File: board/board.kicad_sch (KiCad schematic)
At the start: 13 parts, among them J1 Conn_01x19, J2 Conn_01x19, J3 Conn_01x02, U1 ESP32-WROVER-E, U2 AOZ1280CI

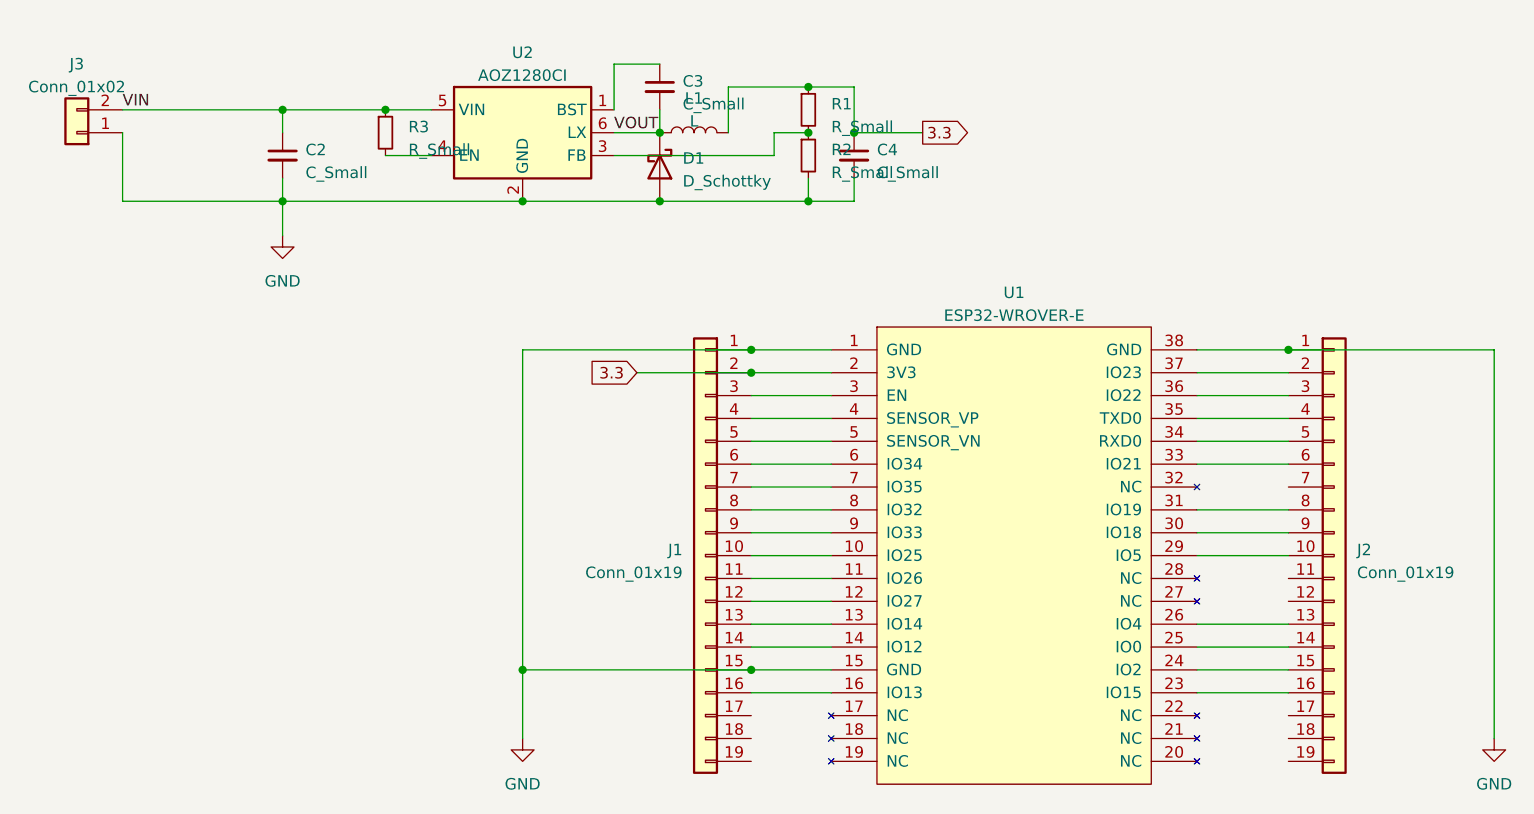
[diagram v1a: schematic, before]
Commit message: dev
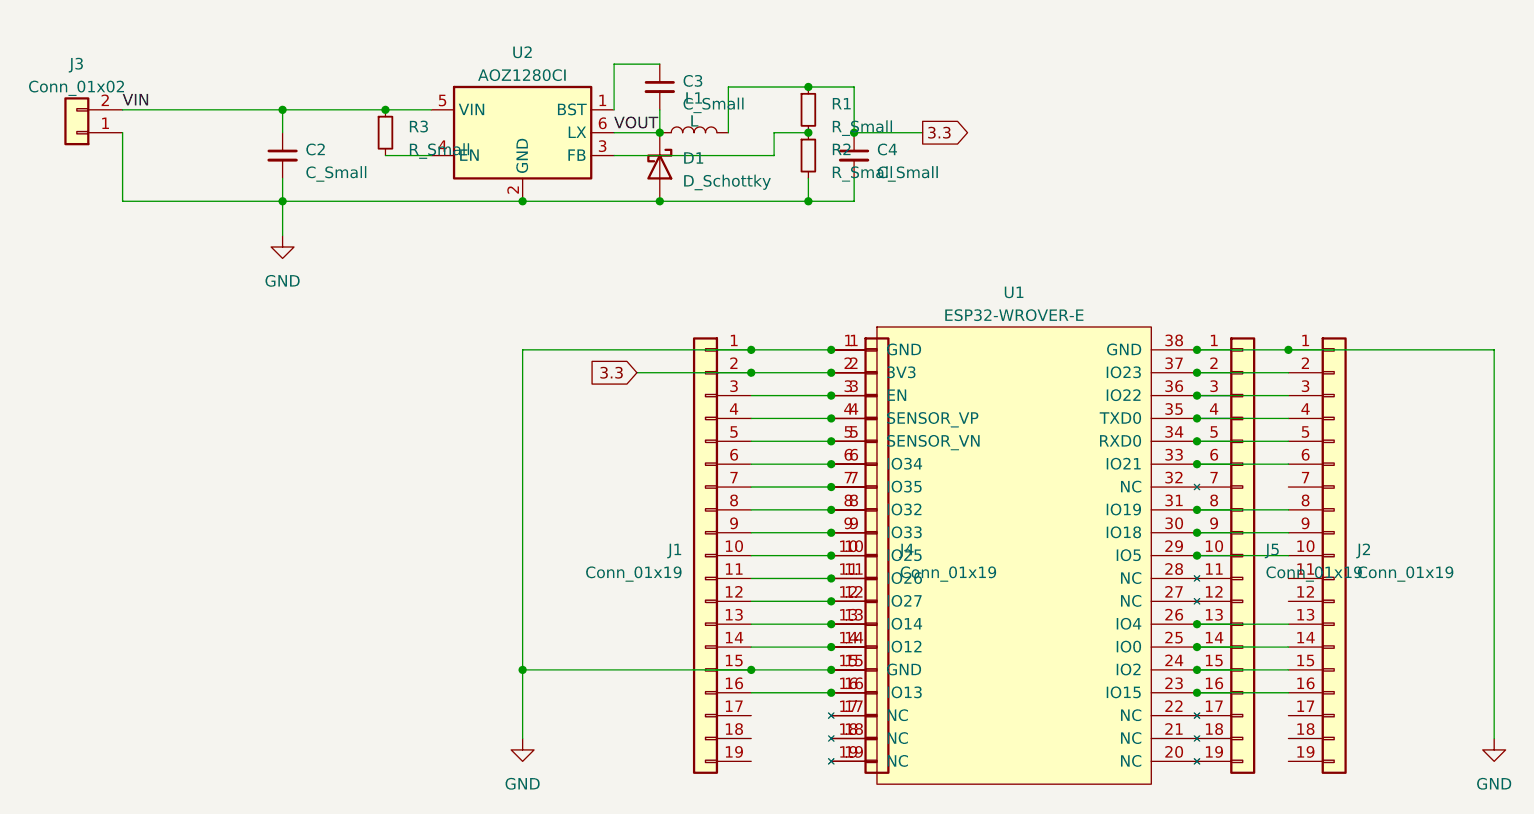
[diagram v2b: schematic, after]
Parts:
- added J4, J5: Conn_01x19, Connector_PinHeader_1.27mm:PinHeader_1x19_P1.27mm_Vertical, symbol Connector_Generic:Conn_01x19
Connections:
- net 3.3: now also J4.2 (Pin_2)
- net GND: now also J4.1 (Pin_1), J4.15 (Pin_15), J5.1 (Pin_1)
- net at J2.10 (Pin_10), U1.29 (IO5): now also J5.10 (Pin_10)
- net at J2.13 (Pin_13), U1.26 (IO4): now also J5.13 (Pin_13)
- net at J2.14 (Pin_14), U1.25 (IO0): now also J5.14 (Pin_14)
- net at J2.15 (Pin_15), U1.24 (IO2): now also J5.15 (Pin_15)
- net at J2.16 (Pin_16), U1.23 (IO15): now also J5.16 (Pin_16)
- net at J2.2 (Pin_2), U1.37 (IO23): now also J5.2 (Pin_2)
- net at J2.3 (Pin_3), U1.36 (IO22): now also J5.3 (Pin_3)
- net at J2.4 (Pin_4), U1.35 (TXD0): now also J5.4 (Pin_4)
- net at J2.5 (Pin_5), U1.34 (RXD0): now also J5.5 (Pin_5)
- net at J2.6 (Pin_6), U1.33 (IO21): now also J5.6 (Pin_6)
- net at J2.8 (Pin_8), U1.31 (IO19): now also J5.8 (Pin_8)
- net at J2.9 (Pin_9), U1.30 (IO18): now also J5.9 (Pin_9)
- net at J1.10 (Pin_10), U1.10 (IO25): now also J4.10 (Pin_10)
- net at J1.11 (Pin_11), U1.11 (IO26): now also J4.11 (Pin_11)
- net at J1.12 (Pin_12), U1.12 (IO27): now also J4.12 (Pin_12)
- net at J1.13 (Pin_13), U1.13 (IO14): now also J4.13 (Pin_13)
- net at J1.14 (Pin_14), U1.14 (IO12): now also J4.14 (Pin_14)
- net at J1.16 (Pin_16), U1.16 (IO13): now also J4.16 (Pin_16)
- net at J1.3 (Pin_3), U1.3 (EN): now also J4.3 (Pin_3)
- net at J1.4 (Pin_4), U1.4 (SENSOR_VP): now also J4.4 (Pin_4)
- net at J1.5 (Pin_5), U1.5 (SENSOR_VN): now also J4.5 (Pin_5)
- net at J1.6 (Pin_6), U1.6 (IO34): now also J4.6 (Pin_6)
- net at J1.7 (Pin_7), U1.7 (IO35): now also J4.7 (Pin_7)
- net at J1.8 (Pin_8), U1.8 (IO32): now also J4.8 (Pin_8)
- net at J1.9 (Pin_9), U1.9 (IO33): now also J4.9 (Pin_9)
- net at U1.17 (NC): now also J4.17 (Pin_17)
- net at U1.18 (NC): now also J4.18 (Pin_18)
- net at U1.19 (NC): now also J4.19 (Pin_19)
- net at U1.20 (NC): now also J5.19 (Pin_19)
- net at U1.21 (NC): now also J5.18 (Pin_18)
- net at U1.22 (NC): now also J5.17 (Pin_17)
- net at U1.27 (NC): now also J5.12 (Pin_12)
- net at U1.28 (NC): now also J5.11 (Pin_11)
- net at U1.32 (NC): now also J5.7 (Pin_7)
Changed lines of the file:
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@@
 (kicad_sch (version 20220904) (generator eeschema)
   (paper "A4")
+  (junction (at 132.08 73.66) (diameter 0) (color 0 0 0 0)
+  )
+  (junction (at 132.08 86.36) (diameter 0) (color 0 0 0 0)
+  )
+  (junction (at 172.72 86.36) (diameter 0) (color 0 0 0 0)
+  )
+  (junction (at 132.08 68.58) (diameter 0) (color 0 0 0 0)
+  )
+  (junction (at 132.08 78.74) (diameter 0) (color 0 0 0 0)
+  )
+  (junction (at 132.08 76.2) (diameter 0) (color 0 0 0 0)
+  )
   (junction (at 113.03 29.21) (diameter 0) (color 0 0 0 0)
   )
   (junction (at 134.62 29.21) (diameter 0) (color 0 0 0 0)
   )
+  (junction (at 172.72 83.82) (diameter 0) (color 0 0 0 0)
+  )
+  (junction (at 172.72 58.42) (diameter 0) (color 0 0 0 0)
+  )
+  (junction (at 132.08 63.5) (diameter 0) (color 0 0 0 0)
+  )
+  (junction (at 172.72 66.04) (diameter 0) (color 0 0 0 0)
+  )
+  (junction (at 172.72 88.9) (diameter 0) (color 0 0 0 0)
+  )
   (junction (at 123.19 55.88) (diameter 0) (color 0 0 0 0)
   )
@@
   (junction (at 123.19 53.34) (diameter 0) (color 0 0 0 0)
   )
+  (junction (at 172.72 76.2) (diameter 0) (color 0 0 0 0)
+  )
+  (junction (at 132.08 53.34) (diameter 0) (color 0 0 0 0)
+  )
+  (junction (at 172.72 73.66) (diameter 0) (color 0 0 0 0)
+  )
   (junction (at 129.54 29.21) (diameter 0) (color 0 0 0 0)
   )
   (junction (at 182.88 53.34) (diameter 0) (color 0 0 0 0)
   )
+  (junction (at 172.72 63.5) (diameter 0) (color 0 0 0 0)
+  )
+  (junction (at 132.08 60.96) (diameter 0) (color 0 0 0 0)
+  )
   (junction (at 113.03 36.83) (diameter 0) (color 0 0 0 0)
   )
+  (junction (at 172.72 55.88) (diameter 0) (color 0 0 0 0)
+  )
+  (junction (at 132.08 71.12) (diameter 0) (color 0 0 0 0)
+  )
+  (junction (at 132.08 88.9) (diameter 0) (color 0 0 0 0)
+  )
   (junction (at 129.54 24.13) (diameter 0) (color 0 0 0 0)
   )
+  (junction (at 132.08 83.82) (diameter 0) (color 0 0 0 0)
+  )
+  (junction (at 172.72 53.34) (diameter 0) (color 0 0 0 0)
+  )
   (junction (at 97.79 88.9) (diameter 0) (color 0 0 0 0)
   )
   (junction (at 71.12 36.83) (diameter 0) (color 0 0 0 0)
   )
+  (junction (at 172.72 71.12) (diameter 0) (color 0 0 0 0)
+  )
+  (junction (at 132.08 58.42) (diameter 0) (color 0 0 0 0)
+  )
+  (junction (at 132.08 91.44) (diameter 0) (color 0 0 0 0)
+  )
+  (junction (at 132.08 55.88) (diameter 0) (color 0 0 0 0)
+  )
+  (junction (at 132.08 81.28) (diameter 0) (color 0 0 0 0)
+  )
   (junction (at 97.79 36.83) (diameter 0) (color 0 0 0 0)
   )
@@
   (junction (at 71.12 26.67) (diameter 0) (color 0 0 0 0)
   )
+  (junction (at 172.72 91.44) (diameter 0) (color 0 0 0 0)
+  )
+  (junction (at 172.72 60.96) (diameter 0) (color 0 0 0 0)
+  )
   (junction (at 123.19 88.9) (diameter 0) (color 0 0 0 0)
+  )
+  (junction (at 132.08 66.04) (diameter 0) (color 0 0 0 0)
   )
   (wire (pts (xy 172.72 91.44) (xy 182.88 91.44))
@@
     (pin "2")
   )
+  (symbol (lib_id "Connector_Generic:Conn_01x19") (at 137.16 76.2 0) (unit 1)
+    (in_bom yes) (on_board yes) (fields_autoplaced)
+    (default_instance (reference "J4") (unit 1) (value "Conn_01x19") (footprint "Connector_PinHeader_1.27mm:PinHeader_1x19_P1.27mm_Vertical"))
+    (property "Reference" "J4" (id 0) (at 139.7 75.565 0)
+      (effects (font (size 1.27 1.27)) (justify left))
+    )
+    (property "Value" "Conn_01x19" (id 1) (at 139.7 78.105 0)
+      (effects (font (size 1.27 1.27)) (justify left))
+    )
+    (property "Footprint" "Connector_PinHeader_1.27mm:PinHeader_1x19_P1.27mm_Vertical" (id 2) (at 137.16 76.2 0)
+      (effects (font (size 1.27 1.27)) hide)
+    )
+    (property "Datasheet" "~" (id 3) (at 137.16 76.2 0)
+      (effects (font (size 1.27 1.27)) hide)
+    )
+    (pin "1")
+    (pin "10")
+    (pin "11")
+    (pin "12")
+    (pin "13")
+    (pin "14")
+    (pin "15")
+    (pin "16")
+    (pin "17")
+    (pin "18")
+    (pin "19")
+    (pin "2")
+    (pin "3")
+    (pin "4")
+    (pin "5")
+    (pin "6")
+    (pin "7")
+    (pin "8")
+    (pin "9")
+  )
   (symbol (lib_id "power:GND") (at 97.79 96.52 0) (unit 1)
     (in_bom yes) (on_board yes) (fields_autoplaced)
@@
     (pin "1")
     (pin "2")
+  )
+  (symbol (lib_id "Connector_Generic:Conn_01x19") (at 177.8 76.2 0) (unit 1)
+    (in_bom yes) (on_board yes) (fields_autoplaced)
+    (default_instance (reference "J5") (unit 1) (value "Conn_01x19") (footprint "Connector_PinHeader_1.27mm:PinHeader_1x19_P1.27mm_Vertical"))
+    (property "Reference" "J5" (id 0) (at 180.34 75.565 0)
+      (effects (font (size 1.27 1.27)) (justify left))
+    )
+    (property "Value" "Conn_01x19" (id 1) (at 180.34 78.105 0)
+      (effects (font (size 1.27 1.27)) (justify left))
+    )
+    (property "Footprint" "Connector_PinHeader_1.27mm:PinHeader_1x19_P1.27mm_Vertical" (id 2) (at 177.8 76.2 0)
+      (effects (font (size 1.27 1.27)) hide)
+    )
+    (property "Datasheet" "~" (id 3) (at 177.8 76.2 0)
+      (effects (font (size 1.27 1.27)) hide)
+    )
+    (pin "1")
+    (pin "10")
+    (pin "11")
+    (pin "12")
+    (pin "13")
+    (pin "14")
+    (pin "15")
+    (pin "16")
+    (pin "17")
+    (pin "18")
+    (pin "19")
+    (pin "2")
+    (pin "3")
+    (pin "4")
+    (pin "5")
+    (pin "6")
+    (pin "7")
+    (pin "8")
+    (pin "9")
   )
   (sheet_instances
@@
       (reference "J3") (unit 1) (value "3.3-26V") (footprint "Custom_Connector:Ninigi AC141R-02P-2.54")
     )
+    (path "/821d4e86-e26e-4f23-8eb8-9a9368942310"
+      (reference "J4") (unit 1) (value "Conn_01x19") (footprint "Connector_PinHeader_1.27mm:PinHeader_1x19_P1.27mm_Vertical")
+    )
+    (path "/f990144d-0bac-40f0-a088-f84ad934828c"
+      (reference "J5") (unit 1) (value "Conn_01x19") (footprint "Connector_PinHeader_1.27mm:PinHeader_1x19_P1.27mm_Vertical")
+    )
     (path "/2242ca84-47e8-48a2-92d3-0266cd11783b"

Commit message: dev
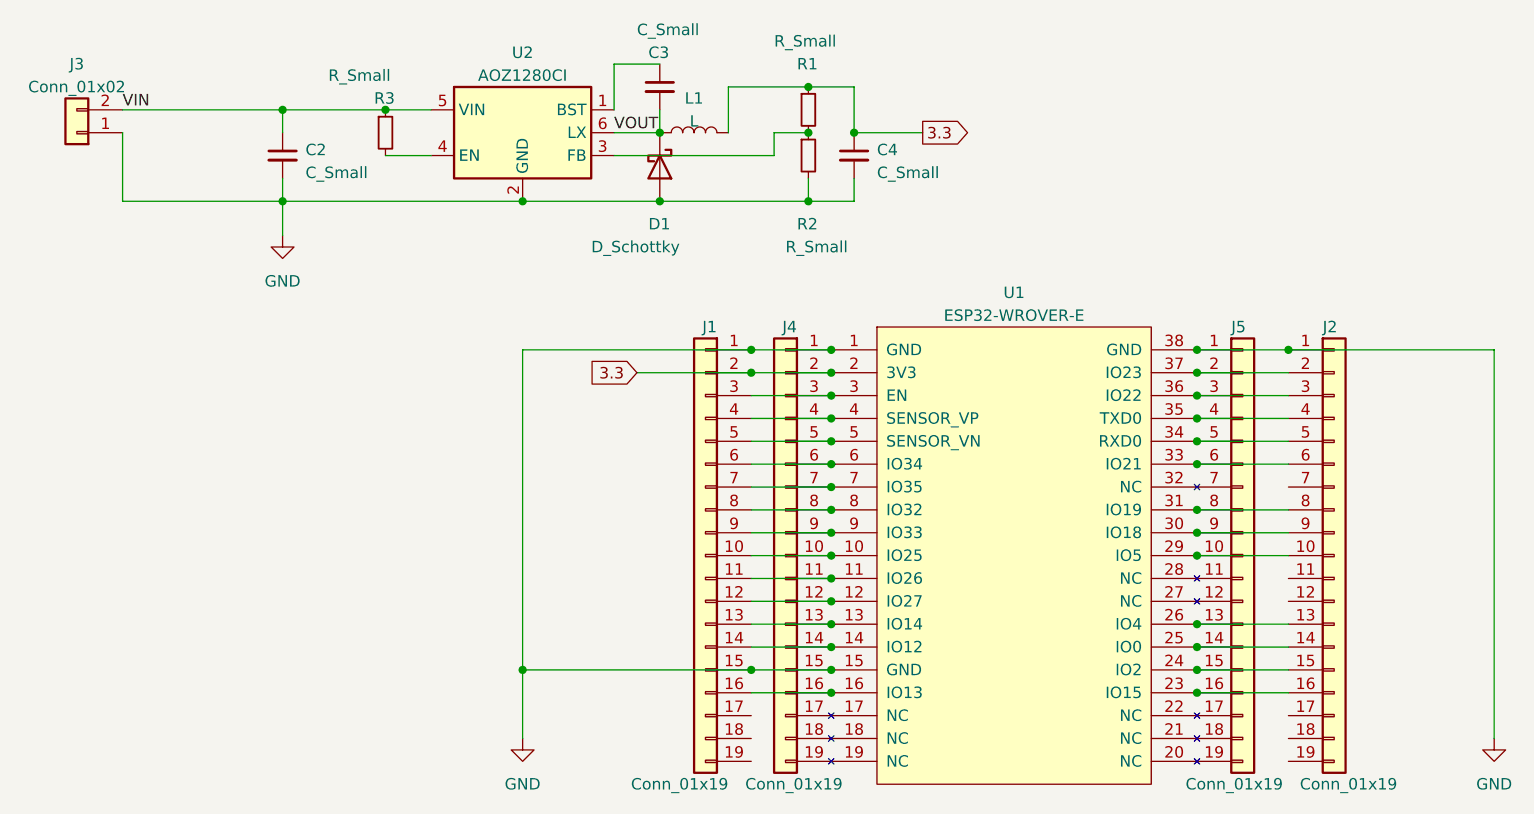
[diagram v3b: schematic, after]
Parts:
- C2: Type (none) -> T491D475K050AT
- J3: Type (none) -> Ninigi AC141R-02P-2.54
- L1: Type (none) -> Walsin WLPN303015M2R2PB
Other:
- moved on the sheet: J4
